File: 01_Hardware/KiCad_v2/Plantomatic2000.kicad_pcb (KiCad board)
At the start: 4 copper layers, 116 x 72 mm, 295 parts, among them J100 TYPE-C-31-M-12, J300 JST_B2B, J600 JST_B2B, J601 JST_B2B, J700 JST_B4B, J701 JST_B4B, J800 Conn_02x03_Odd_Even, J801 JST_B2B, J802 JST_B2B, J803 JST_B2B, J804 Conn_02x05_Odd_Even, J805 JST_B2B, J806 JST_B2B, J807 JST_B2B, J808 JST_B2B, Q100 UMH3N, Q113 CSD17313Q2, Q200 SI7615DN-T1-GE3, Q201 SI7615DN-T1-GE3, Q202 DMP6050SSD-13, Q203 IRLML2402TRPBF, Q204 SI7615DN-T1-GE3, Q205 IRLML2402TRPBF, Q300 BSS314PEH6327, Q301 IRLML2402TRPBF, Q500 IRLML2402TRPBF, Q600 STN3NF06L, Q601 STN3NF06L, Q700 BSS314PEH6327, Q701 BSS314PEH6327, Q702 IRLML2402TRPBF, Q703 IRLML2402TRPBF, SW800 SW_Push, SW801 SW_Push, U100 USBLC6-2P6, U101 CP2102N-A02-GQFN24R, U104 TPS61287RZPR, U200 CYPD3177-24LQ, U300 BQ25892, U403 XC6220B331MR-G, U404 XC6220B331MR-G, U405 LM1085IS-12/NOPB, U406 LM1085IS-12/NOPB, U500 DS3231M, U501 ESP32-WROOM-32E-N4, U502 AT24CS01-SSHM

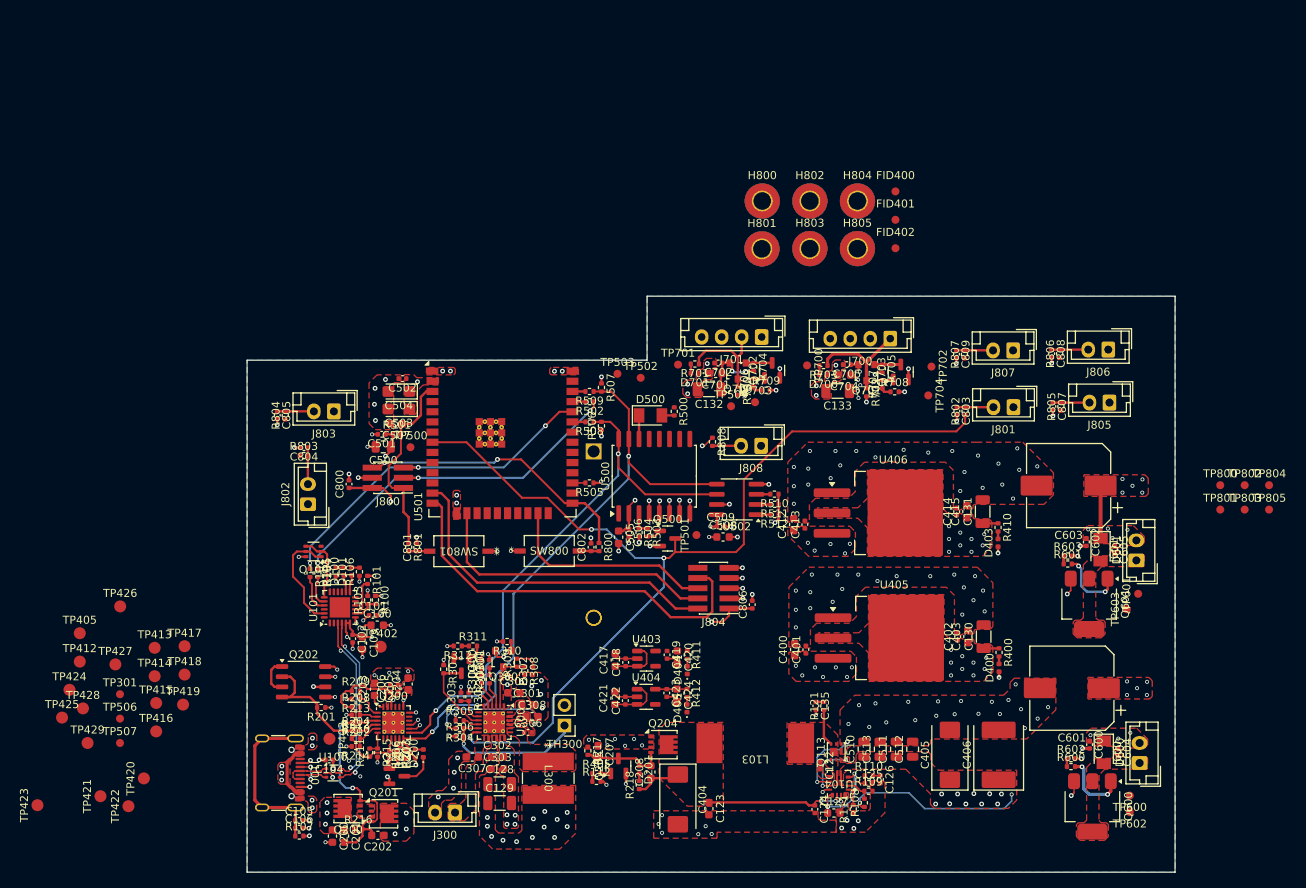
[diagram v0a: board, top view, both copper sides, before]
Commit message: Hardware for manufacturing v0.2
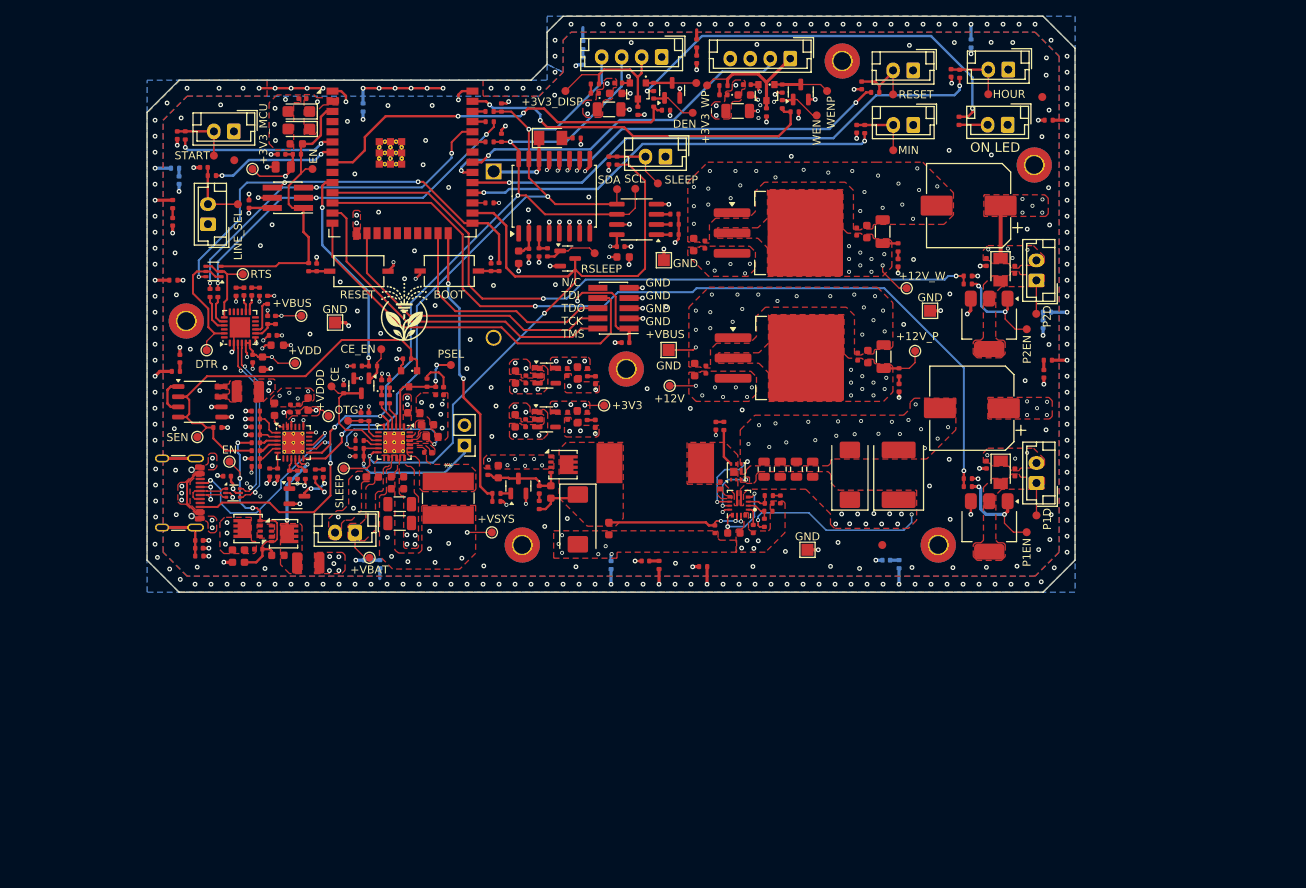
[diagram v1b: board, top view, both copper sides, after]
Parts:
- removed the G*** at (401.6, 225.9)
- removed TP415, TP416, TP417, TP418, TP421, TP425: TestPoint_Small, TestPoint:TestPoint_Pad_D1.5mm
- added +VBAT: TestPoint_Small, TestPoint:TestPoint_Pad_D1.0mm, F.Cu at (126.9, 138.6)
- added C407: 4.7nF, Capacitor_SMD:C_0402_1005Metric, F.Cu at (211.2, 115.6)
- added C408: 4.7nF, Capacitor_SMD:C_0402_1005Metric, F.Cu at (161.4, 139.0)
- added C409: 4.7nF, Capacitor_SMD:C_0402_1005Metric, F.Cu at (103.2, 113.7)
- added C410: 4.7nF, Capacitor_SMD:C_0402_1005Metric, F.Cu at (102.3, 96.6)
- added C411: 4.7nF, Capacitor_SMD:C_0402_1005Metric, F.Cu at (167.8, 76.3)
- added C416: 4.7nF, Capacitor_SMD:C_0402_1005Metric, B.Cu at (211.1, 109.4)
- added C425: 4.7nF, Capacitor_SMD:C_0402_1005Metric, B.Cu at (191.5, 138.9)
- added C426: 4.7nF, Capacitor_SMD:C_0402_1005Metric, B.Cu at (126.7, 138.9)
- added C427: 4.7nF, Capacitor_SMD:C_0402_1005Metric, B.Cu at (103.1, 91.4)
- added C428: 4.7nF, Capacitor_SMD:C_0402_1005Metric, B.Cu at (153.6, 76.5)
- added F400: Polyfuse_Small, Fuse:Fuse_1210_3225Metric, F.Cu at (119.2, 139.2)
- added F401: Polyfuse_Small, Fuse:Fuse_1210_3225Metric, F.Cu at (111.7, 117.8)
- added G***: LOGO, LOGO, F.Cu at (131.2, 108.0)
- added G***: LOGO, LOGO, B.Cu at (162.3, 129.2)
- added GND: TestPoint, TestPoint:TestPoint_Pad_1.5x1.5mm, F.Cu at (197.0, 107.7)
- added GND: TestPoint, TestPoint:TestPoint_Pad_1.5x1.5mm, F.Cu at (163.7, 101.4)
- added GND: TestPoint, TestPoint:TestPoint_Pad_1.5x1.5mm, F.Cu at (164.3, 112.6)
- added GND: TestPoint, TestPoint:TestPoint_Pad_1.5x1.5mm, F.Cu at (181.7, 137.6)
- added GND: TestPoint, TestPoint:TestPoint_Pad_1.5x1.5mm, F.Cu at (122.6, 109.2)
- added R401: 22R, Resistor_SMD:R_0402_1005Metric, F.Cu at (211.7, 113.9)
- added R402: 511K, Resistor_SMD:R_0402_1005Metric, F.Cu at (211.8, 83.9)
- added R403: 511K, Resistor_SMD:R_0402_1005Metric, F.Cu at (168.6, 139.7)
- added R404: 511K, Resistor_SMD:R_0402_1005Metric, F.Cu at (102.4, 103.9)
- added R406: 511K, Resistor_SMD:R_0402_1005Metric, B.Cu at (157.1, 139.5)
- added R407: 22R, Resistor_SMD:R_0402_1005Metric, F.Cu at (163.1, 139.5)
- added R408: 22R, Resistor_SMD:R_0402_1005Metric, F.Cu at (102.7, 115.3)
- added R409: 22R, Resistor_SMD:R_0402_1005Metric, F.Cu at (102.3, 94.4)
- added R413: 22R, Resistor_SMD:R_0402_1005Metric, F.Cu at (167.8, 74.3)
- added R414: 22R, Resistor_SMD:R_0402_1005Metric, B.Cu at (211.6, 107.9)
- added R415: 22R, Resistor_SMD:R_0402_1005Metric, B.Cu at (193.1, 139.4)
- added R416: 22R, Resistor_SMD:R_0402_1005Metric, B.Cu at (128.2, 139.4)
- added R417: 22R, Resistor_SMD:R_0402_1005Metric, B.Cu at (102.6, 89.9)
- added R418: 22R, Resistor_SMD:R_0402_1005Metric, B.Cu at (153.6, 74.5)
- added R419: 511K, Resistor_SMD:R_0402_1005Metric, B.Cu at (202.1, 74.3)
- added R420: 511K, Resistor_SMD:R_0402_1005Metric, B.Cu at (126.1, 82.3)
- +12V: renamed from TP424; footprint TestPoint:TestPoint_Pad_D1.5mm -> TestPoint:TestPoint_Pad_D1.0mm
- +12V_P: renamed from TP426; footprint TestPoint:TestPoint_Pad_D1.5mm -> TestPoint:TestPoint_Pad_D1.0mm
- +12V_W: renamed from TP427; footprint TestPoint:TestPoint_Pad_D1.5mm -> TestPoint:TestPoint_Pad_D1.0mm
- +3V3: renamed from TP429; footprint TestPoint:TestPoint_Pad_D1.5mm -> TestPoint:TestPoint_Pad_D1.0mm
- +3V3_MCU: renamed from TP428; footprint TestPoint:TestPoint_Pad_D1.5mm -> TestPoint:TestPoint_Pad_D1.0mm
- +VBUS: renamed from TP403; footprint TestPoint:TestPoint_Pad_D1.5mm -> TestPoint:TestPoint_Pad_D1.0mm
- +VDD: renamed from TP402; footprint TestPoint:TestPoint_Pad_D1.5mm -> TestPoint:TestPoint_Pad_D1.0mm
- +VDDD: renamed from TP413; footprint TestPoint:TestPoint_Pad_D1.5mm -> TestPoint:TestPoint_Pad_D1.0mm
- +VSYS: renamed from TP423; footprint TestPoint:TestPoint_Pad_D1.5mm -> TestPoint:TestPoint_Pad_D1.0mm
- DTR: renamed from TP405; footprint TestPoint:TestPoint_Pad_D1.5mm -> TestPoint:TestPoint_Pad_D1.0mm
- EN: renamed from TP419; footprint TestPoint:TestPoint_Pad_D1.5mm -> TestPoint:TestPoint_Pad_D1.0mm
- OTG: renamed from TP420; footprint TestPoint:TestPoint_Pad_D1.5mm -> TestPoint:TestPoint_Pad_D1.0mm
- RTS: renamed from TP412; footprint TestPoint:TestPoint_Pad_D1.5mm -> TestPoint:TestPoint_Pad_D1.0mm
- SEN: renamed from TP414; footprint TestPoint:TestPoint_Pad_D1.5mm -> TestPoint:TestPoint_Pad_D1.0mm
- SLEEP: renamed from TP422; footprint TestPoint:TestPoint_Pad_D1.5mm -> TestPoint:TestPoint_Pad_D1.0mm
- moved START 135.3 mm to (107.5, 88.3)
- moved LINE_SEL 128.6 mm to (110.5, 94.4)
- moved +12V_W 109.5 mm to (194.1, 104.9)
- moved +12V_P 104.4 mm to (195.1, 112.8)
- moved +12V 84.1 mm to (164.4, 117.1)
- moved FID400 82.7 mm to (110.0, 88.9)
- moved SLEEP 79.8 mm to (162.9, 91.8)
- moved +3V3 77.1 mm to (156.2, 119.5)
- moved H801 72.5 mm to (104.0, 109.0)
- moved +3V3_MCU 70.7 mm to (112.3, 90.0)
- moved RESET 70.0 mm to (192.3, 80.7)
- moved +VSYS 66.2 mm to (142.2, 135.4)
- moved MIN 62.8 mm to (192.4, 87.7)
- moved PSEL 62.8 mm to (137.1, 114.5)
- moved HOUR 60.2 mm to (204.2, 80.7)
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- renumbered TP509 to +3V3_DISP, TP700 to +3V3_WP, TP506 to CE, TP301 to CE_EN, TP703 to DEN, TP701 to DENP, TP500 to EN, TP804 to HOUR, TP801 to LINE_SEL, TP803 to MIN, TP600 to P1D, TP602 to P1EN, TP601 to P2D, TP603 to P2EN, TP507 to PSEL, TP805 to RESET, TP501 to RSLEEP, TP502 to SCL, TP503 to SDA, TP800 to SLEEP, TP802 to START, TP704 to WEN, TP702 to WENP
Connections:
- net /DISPLAY_AND_WATER_ENABLE/WATER_SENSOR_EN renamed /MICROCONTROLLER/WATER_EN
- net Net-(J100-SHIELD) renamed /USB_C_TO_SERIAL/shield
- C202 pad 1: +5V -> /USB_C_POWER_DELIVERY/fuse_5A
- Q201 pad 5: +5V -> /USB_C_POWER_DELIVERY/fuse_5A
- Q202 pad 7: +5V -> /USB_C_POWER_DELIVERY/Fuse_1A
- Q202 pad 8: +5V -> /USB_C_POWER_DELIVERY/Fuse_1A
- R112 pad 1: /DC_DC_REGULATORS/BOOST_ENABLE -> /MICROCONTROLLER/BOOST_EN
- R311 pad 1: /BATTERY_MANAGEMENT_IC/CHARGE_ENABLE -> /MICROCONTROLLER/CHARGE_EN
- R312 pad 1: /BATTERY_MANAGEMENT_IC/CHARGE_ENABLE -> /MICROCONTROLLER/CHARGE_EN
- R405 pad 1: /DC_DC_REGULATORS/BOOST_ENABLE -> /MICROCONTROLLER/BOOST_EN
- R803 pad 1: /CONNECTORS/SELECT_LINE_BUTTON_PIN -> /MICROCONTROLLER/SELECT_LINE_PIN
- R804 pad 1: ESP_TMS -> /MICROCONTROLLER/START_PIN
- R805 pad 1: /CONNECTORS/MIN_BUTTON_PIN -> /MICROCONTROLLER/MIN_PIN
- R806 pad 1: /CONNECTORS/HOUR_BUTTON_PIN -> /MICROCONTROLLER/HOUR_PIN
- R807 pad 1: /CONNECTORS/RESET_BUTTON_PIN -> /MICROCONTROLLER/RESET_PIN
- U200 pad 11: +5V -> /USB_C_POWER_DELIVERY/fuse_5A
- U501 pad 10: /CONNECTORS/SELECT_LINE_BUTTON_PIN -> /MICROCONTROLLER/CHARGE_EN
- U501 pad 11: /CONNECTORS/MIN_BUTTON_PIN -> /MICROCONTROLLER/PUMP2_EN
- U501 pad 12: /CONNECTORS/HOUR_BUTTON_PIN -> /MICROCONTROLLER/PUMP1_EN
- U501 pad 24: /MICROCONTROLLER/DISP_EN -> /MICROCONTROLLER/BOOST_EN
- U501 pad 26: /MICROCONTROLLER/WATER_SIG -> WAKE_SLEEP
- U501 pad 28: /BATTERY_MANAGEMENT_IC/CHARGE_ENABLE -> /MICROCONTROLLER/MIN_PIN
- U501 pad 29: unconnected-(U501-IO5-Pad29) -> /MICROCONTROLLER/HOUR_PIN
- U501 pad 30: /MICROCONTROLLER/PUMP2_EN -> /MICROCONTROLLER/RESET_PIN
- U501 pad 31: /MICROCONTROLLER/PUMP1_EN -> /MICROCONTROLLER/WATER_SIG
- U501 pad 6: /DC_DC_REGULATORS/BOOST_ENABLE -> /MICROCONTROLLER/START_PIN
- U501 pad 7: unconnected-(U501-IO35-Pad7) -> /MICROCONTROLLER/SELECT_LINE_PIN
- U501 pad 8: WAKE_SLEEP -> /MICROCONTROLLER/DISP_EN
- U501 pad 9: /CONNECTORS/RESET_BUTTON_PIN -> unconnected-(U501-IO33-Pad9)
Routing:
- net /MICROCONTROLLER/PUMP1_EN: track 1.00 -> 108.1 mm, vias 0 -> 2
- net /MICROCONTROLLER/PUMP2_EN: track 1.00 -> 90.3 mm, vias 0 -> 2
- net /MICROCONTROLLER/HOUR_PIN: track 0.00 -> 67.2 mm, vias 0 -> 2
- net /MICROCONTROLLER/RESET_PIN: track 0.00 -> 57.0 mm, vias 0 -> 2
- net /MICROCONTROLLER/MIN_PIN: track 0.00 -> 52.7 mm, vias 0 -> 2
- net /MICROCONTROLLER/DISP_EN: track 1.38 -> 47.6 mm, vias 0 -> 2
- net +3V3: track 14.1 -> 59.3 mm, vias 3 -> 8
- net /MICROCONTROLLER/WATER_EN: track 1.33 -> 45.5 mm, vias 0 -> 2
- net /MICROCONTROLLER/WATER_SIG: track 0.00 -> 43.1 mm, vias 0 -> 1
- net /USB_C_TO_SERIAL/shield: track 21.3 -> 59.8 mm, vias 0 -> 168
- net /BATTERY_MANAGEMENT_IC/VBUS_FET_SAFE_EN: track 17.4 -> 54.0 mm
- net /MICROCONTROLLER/BOOST_EN: track 0.00 -> 36.2 mm, vias 0 -> 2
- net WAKE_SLEEP: track 126.8 -> 92.9 mm, vias 3 -> 2
- net GND: track 93.7 -> 124.1 mm, vias 188 -> 312
- net /MICROCONTROLLER/CHARGE_EN: track 0.00 -> 27.3 mm, vias 0 -> 2
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- added copper zone on F.Cu, net +3V3
- added copper zone on In2.Cu, net +VDDD
- added copper zone on F.Cu, net /BATTERY_MANAGEMENT_IC/PMID
- added copper zone on F.Cu, net /USB_C_POWER_DELIVERY/Fuse_1A
- added copper zone on F.Cu, net /USB_C_POWER_DELIVERY/fuse_5A
- added copper zone on B.Cu, net /USB_C_TO_SERIAL/shield
- added copper zone on F.Cu, net /USB_C_TO_SERIAL/shield
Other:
- outline, holes or cut-outs redrawn
- board text added: "+3V3"
- board text added: "+VBAT"
- board text added: "BOOT"
- board text added: "CR2032"
- board text added: "GND"
- board text added: "GND GND GND GND +VBUS"
- board text added: "IO2: BOOST_ENABLE IO4: WAKE_SLEEP IO5: HOURS IO17: MINUTES IO18: EXTERNAL_RESET IO19: WATER_SIGNAL IO23: WATER_SENSOR_ENABLE IO25: BATTERY CHARGE ENABLE IO26: PUMP_2_ENABLE IO27: PUMP_1_ENABLE IO32: DISPLAY_ENABLE IO34: START_BUTTON IO35: SELECT_LINE"
- board text added: "N/C TDI TDO TCK TMS"
- board text added: "ON LED"
- board text added: "Plantomatic v0.2 20251116"
- board text added: "RESET"
- board text added: "SCL"
- board text added: "SDA"
- board text added: "SIG"
- board text removed: "Plantomatic2000 v0.1 20250625"
